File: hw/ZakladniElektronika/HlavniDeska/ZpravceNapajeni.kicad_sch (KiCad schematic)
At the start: 16 parts, among them Q1 Q_PMOS_DGS, Q10 Q_PMOS_DGS

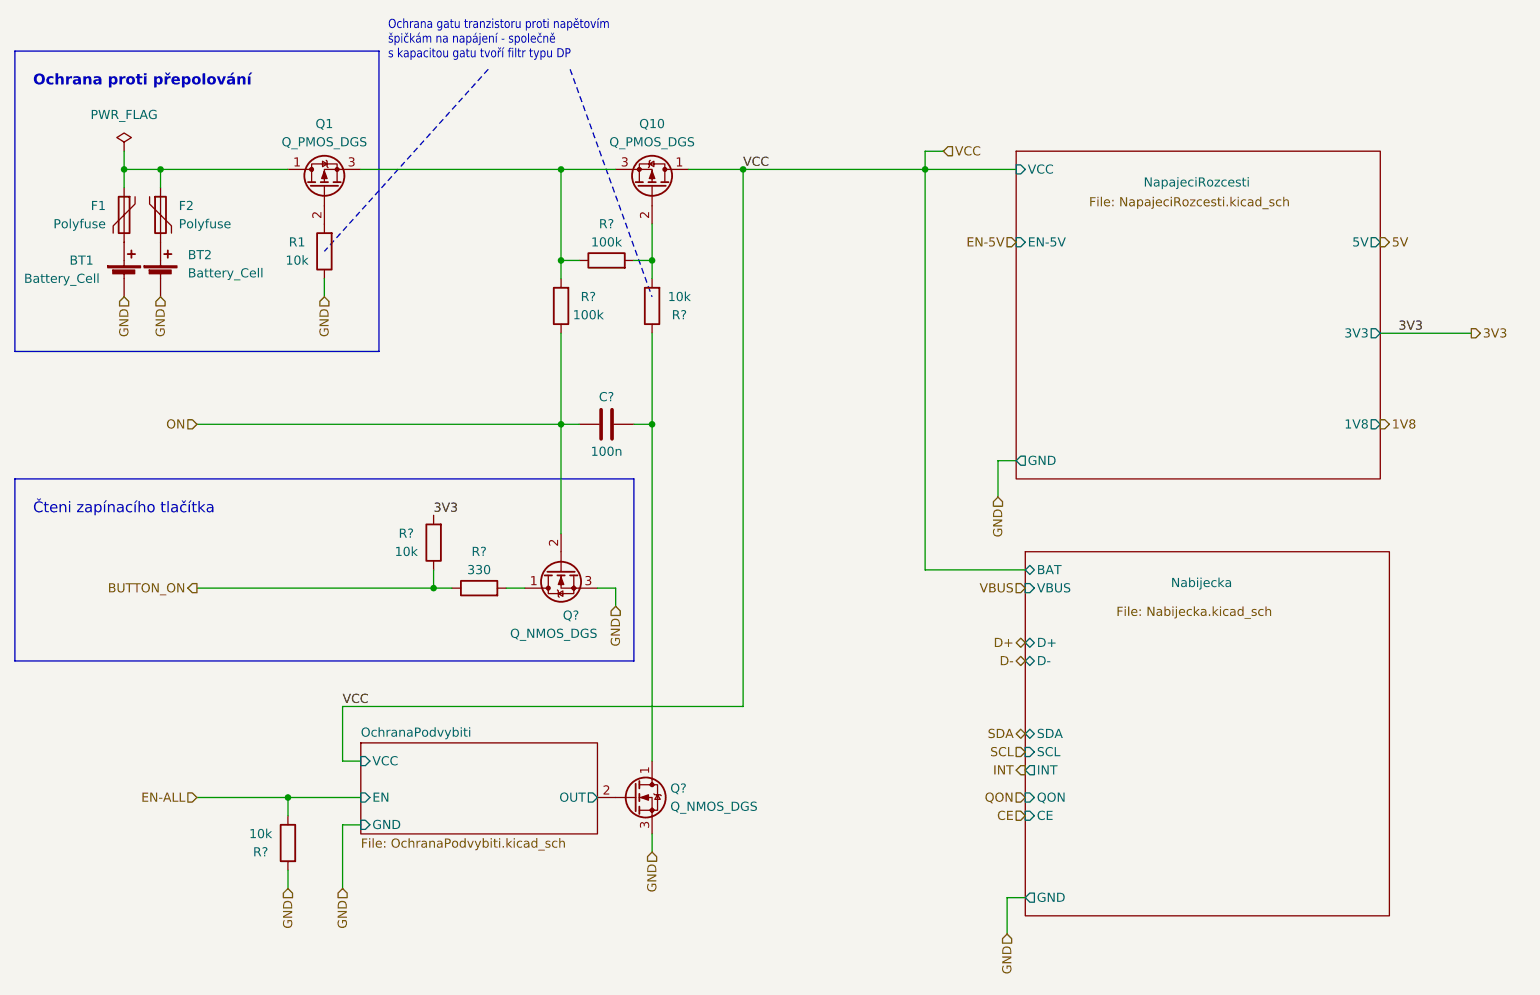
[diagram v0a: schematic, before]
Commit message: Zaciame psat
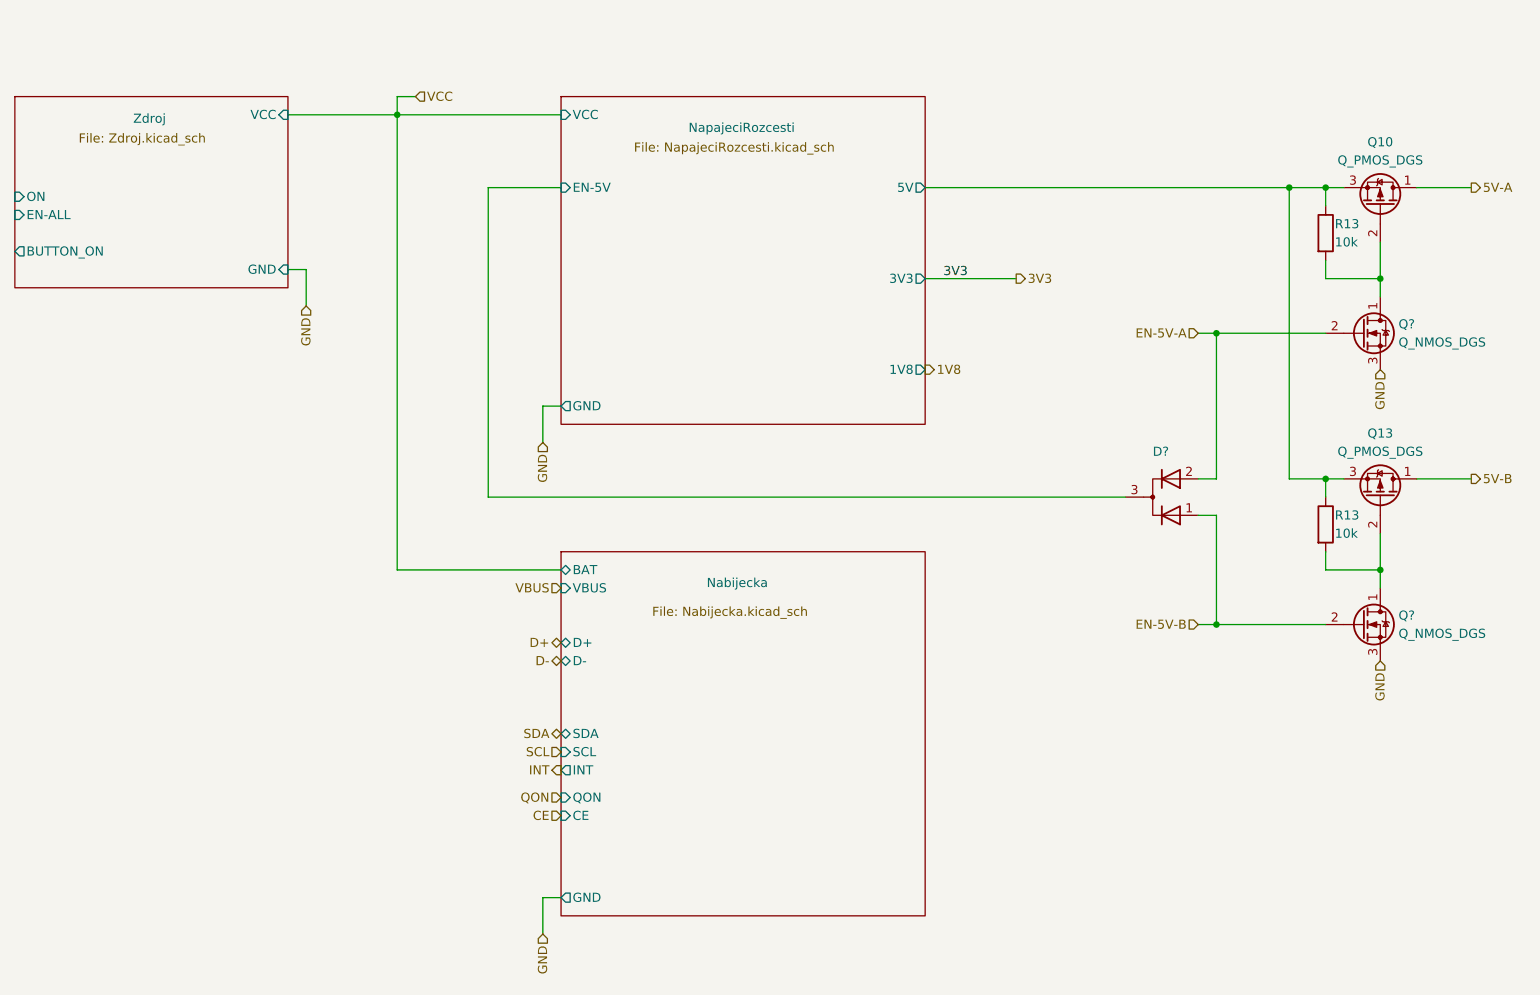
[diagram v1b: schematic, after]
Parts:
- removed BT1, BT2: Battery_Cell, symbol Device:Battery_Cell
- removed C?: 100n, Capacitor_SMD:C_0402_1005Metric, symbol Device:C
- removed F1, F2: Polyfuse, Inductor_SMD:L_1206_3216Metric, symbol Device:Polyfuse
- removed Q1: Q_PMOS_DGS, RBCX:JMSL0302AU, symbol Device:Q_PMOS_DGS
- removed Q? (x2): Q_NMOS_DGS, Package_TO_SOT_SMD:SOT-723, symbol Device:Q_NMOS_DGS
- removed R1, R? (x3): 10k, Capacitor_SMD:C_0201_0603Metric, symbol Device:R
- removed R? (x2): 100k, Capacitor_SMD:C_0201_0603Metric, symbol Device:R
- removed R?: 330, Capacitor_SMD:C_0201_0603Metric, symbol Device:R
- added D?: D_Dual_CommonCathode_AAK_Parallel, Package_TO_SOT_SMD:SOT-723, symbol Device:D_Dual_CommonCathode_AAK_Parallel
- added Q13: Q_PMOS_DGS, RBCX:JMSL0302AU, symbol Device:Q_PMOS_DGS
- added Q? (x2): Q_NMOS_DGS, Package_TO_SOT_SMD:SOT-723, symbol Device:Q_NMOS_DGS
- added R13 (x2): 10k, Resistor_SMD:R_0402_1005Metric, symbol Device:R
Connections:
- net GND: now also Q?.3 (S), Q?.3 (S)
- net VCC: no longer Q10.1 (D)
- net NapajeciRozcesti/5V: now reaches Q10.3 (S)
- net NapajeciRozcesti/5V: now also Q13.3 (S), R13.1, R13.1
- net at Q10.2 (G): now also Q?.1 (D), R13.2
- new net: Q13.2 (G), Q?.1 (D), R13.2
- new net 5V-A: Q10.1 (D)
- new net 5V-B: Q13.1 (D)
- new net EN-5V-A: D?.2 (K), Q?.2 (G)
- new net EN-5V-B: D?.1 (K), Q?.2 (G)
- new net NapajeciRozcesti/EN-5V: D?.3 (A)
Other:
- removed sheet OchranaPodvybiti
- added sheet Zdroj (Zdroj.kicad_sch)
- note removed: "Ochrana gatu tranzistoru proti napětovím špičkám na napájení - společně s kapacitou gatu tvoří filtr typu DP"
- note removed: "Ochrana proti přepolování"
- note removed: "Čteni zapínacího tlačítka"

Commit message: Zavazbení zapínání
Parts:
- Q? (x2): footprint Package_TO_SOT_SMD:SOT-723 -> Package_TO_SOT_SMD:SOT-23; LCSC C2941617 -> C10487
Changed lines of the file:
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@@
       (effects (font (size 1.27 1.27)) (justify left))
     )
-    (property "Footprint" "Package_TO_SOT_SMD:SOT-723" (at 243.84 109.22 0)
+    (property "Footprint" "Package_TO_SOT_SMD:SOT-23" (at 243.84 109.22 0)
       (effects (font (size 1.27 1.27)) hide)
     )
-    (property "Datasheet" "https://datasheet.lcsc.com/lcsc/2004141706_Jiangsu-Changjing-Electronics-Technology-Co---Ltd--2SK3541_C504051.pdf" (at 238.76 111.76 0)
+    (property "Datasheet" "https://datasheet.lcsc.com/lcsc/1808272021_Vishay-Intertech-SI2301CDS-T1-GE3_C10487.pdf" (at 238.76 111.76 0)
       (effects (font (size 1.27 1.27)) hide)
     )
-    (property "LCSC" "C2941617" (at 238.76 111.76 0)
+    (property "LCSC" "C10487" (at 238.76 111.76 0)
       (effects (font (size 1.27 1.27)) hide)
     )
@@
       (effects (font (size 1.27 1.27)) (justify left))
     )
-    (property "Footprint" "Package_TO_SOT_SMD:SOT-723" (at 243.84 68.58 0)
+    (property "Footprint" "Package_TO_SOT_SMD:SOT-23" (at 243.84 68.58 0)
       (effects (font (size 1.27 1.27)) hide)
     )
-    (property "Datasheet" "https://datasheet.lcsc.com/lcsc/2004141706_Jiangsu-Changjing-Electronics-Technology-Co---Ltd--2SK3541_C504051.pdf" (at 238.76 71.12 0)
+    (property "Datasheet" "https://datasheet.lcsc.com/lcsc/1808272021_Vishay-Intertech-SI2301CDS-T1-GE3_C10487.pdf" (at 238.76 71.12 0)
       (effects (font (size 1.27 1.27)) hide)
     )
-    (property "LCSC" "C2941617" (at 238.76 71.12 0)
+    (property "LCSC" "C10487" (at 238.76 71.12 0)
       (effects (font (size 1.27 1.27)) hide)
     )
